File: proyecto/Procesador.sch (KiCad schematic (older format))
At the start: 16 parts

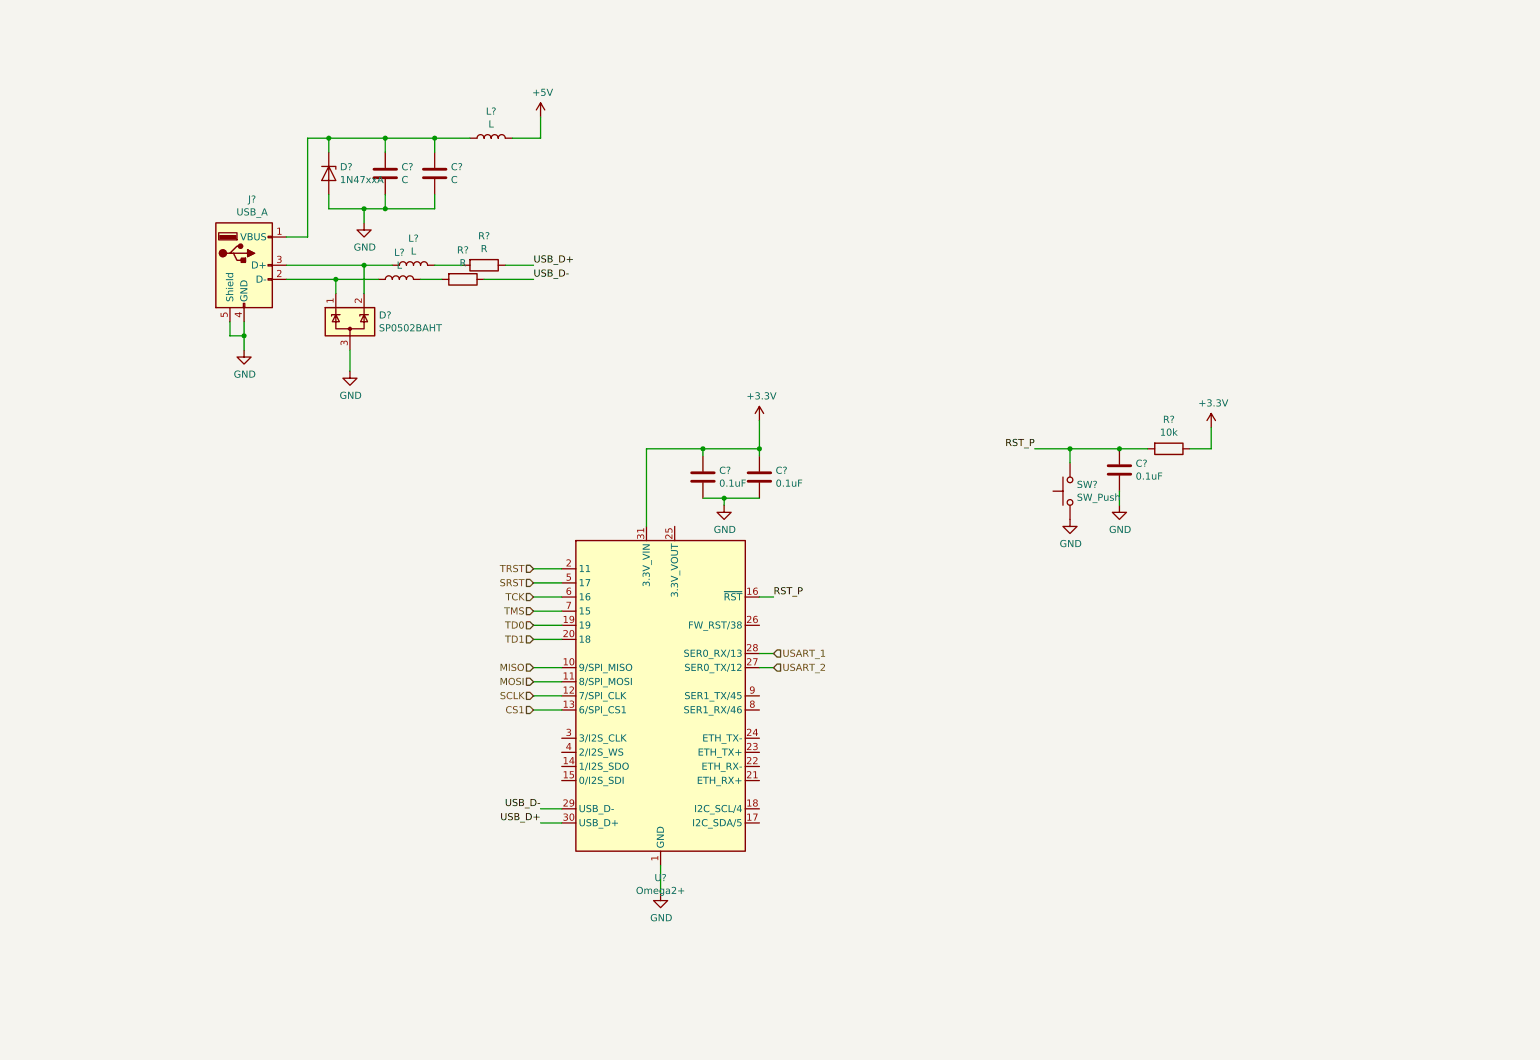
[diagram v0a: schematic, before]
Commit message: Add files via upload
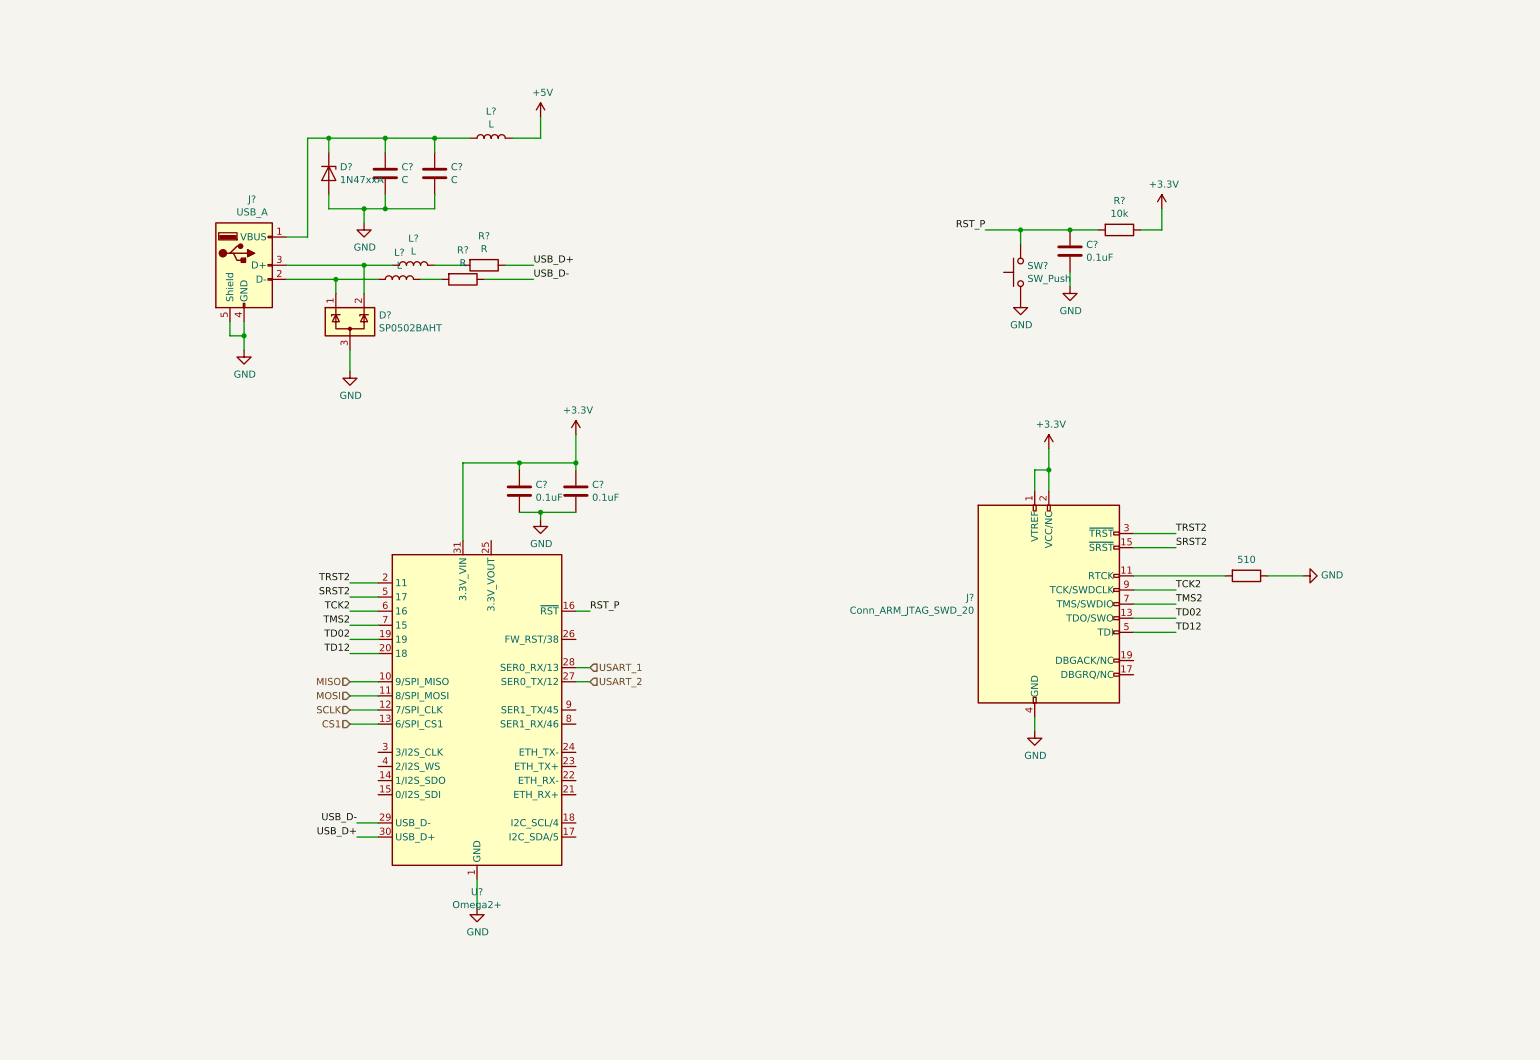
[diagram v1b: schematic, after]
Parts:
- added J?: Conn_ARM_JTAG_SWD_20, symbol Connector:Conn_ARM_JTAG_SWD_20
- added R?: 510, symbol Device:R
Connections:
- net +3V3: now also J?.1 (VTREF), J?.2 (VCC/NC)
- net GND: now also J?.10 (GND), J?.12 (GND), J?.14 (GND), J?.16 (GND), J?.18 (GND), J?.20 (GND), J?.4 (GND), J?.6 (GND), J?.8 (GND), R?.1
- net SRST renamed SRST2
- net SRST2: now also J?.15 (~SRST~)
- net TCK renamed TCK2
- net TCK2: now also J?.9 (TCK/SWDCLK)
- net TD0 renamed TD02
- net TD02: now also J?.13 (TDO/SWO)
- net TD1 renamed TD12
- net TD12: now also J?.5 (TDI)
- net TMS renamed TMS2
- net TMS2: now also J?.7 (TMS/SWDIO)
- net TRST renamed TRST2
- net TRST2: now also J?.3 (~TRST~)
- new net: J?.11 (RTCK), R?.2
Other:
- moved on the sheet: C?, R?, SW?, U?

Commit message: Add files via upload
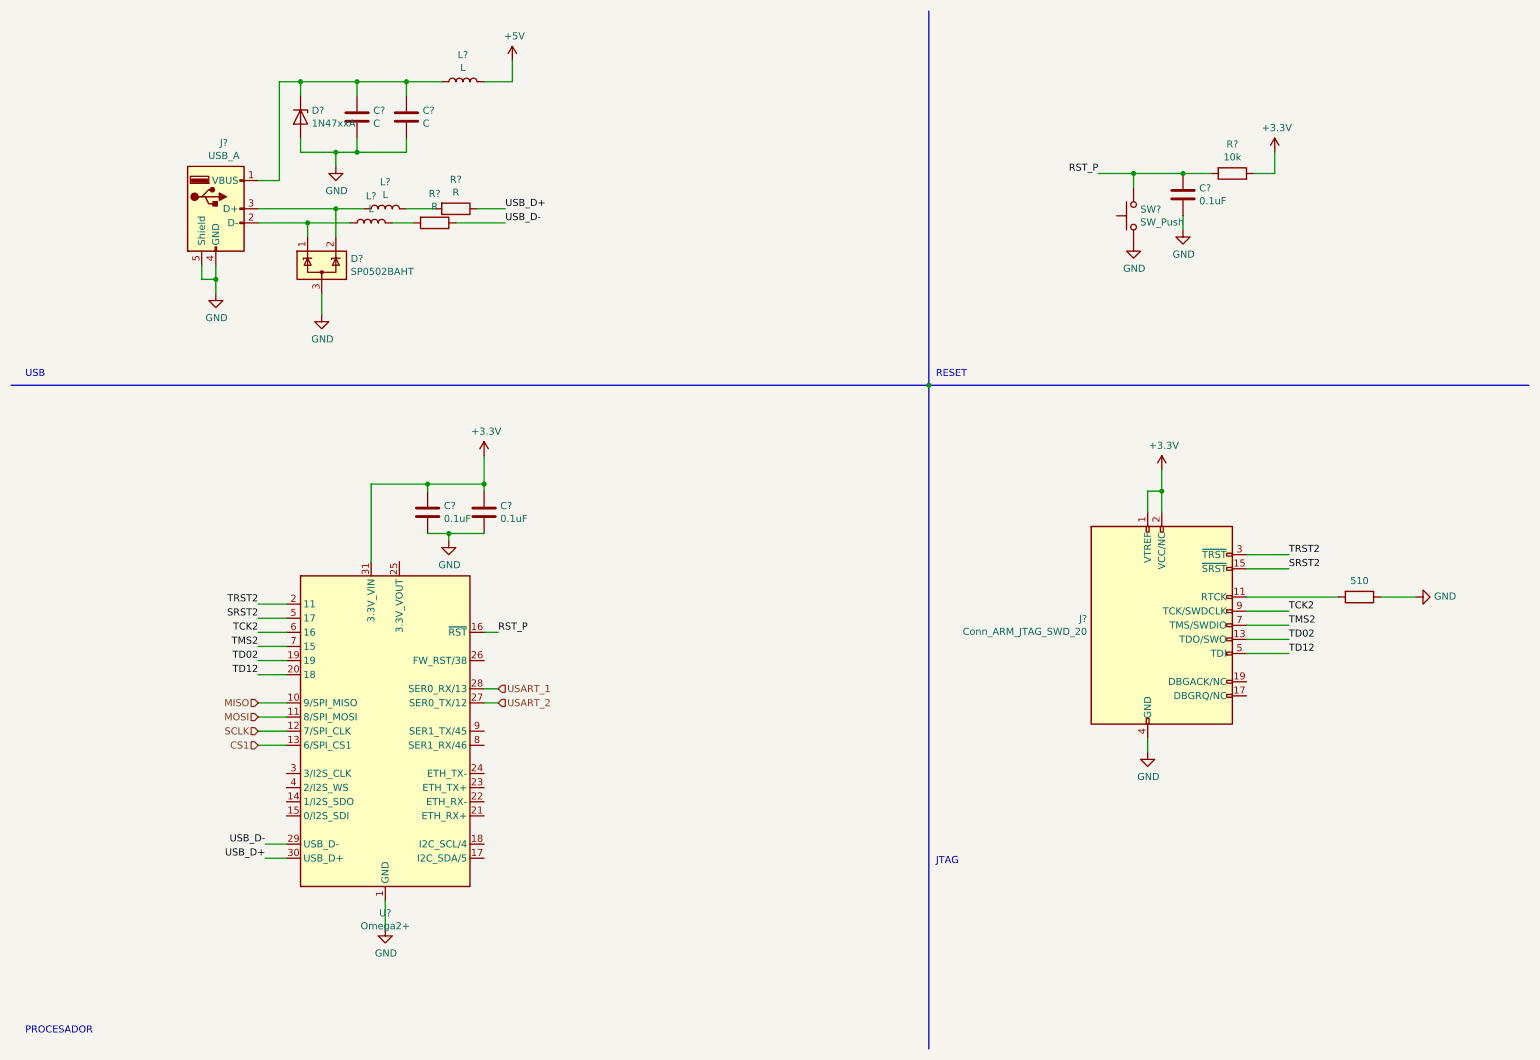
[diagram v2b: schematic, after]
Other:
- note added: "JTAG"
- note added: "PROCESADOR"
- note added: "RESET"
- note added: "USB"
- moved on the sheet: C?, D?, J?, L?, R?, SW?, U?
